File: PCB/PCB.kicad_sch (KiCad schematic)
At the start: 10 parts, among them J3 Conn_02x04_Odd_Even, J5 Conn_02x04_Odd_Even, U2 LM358

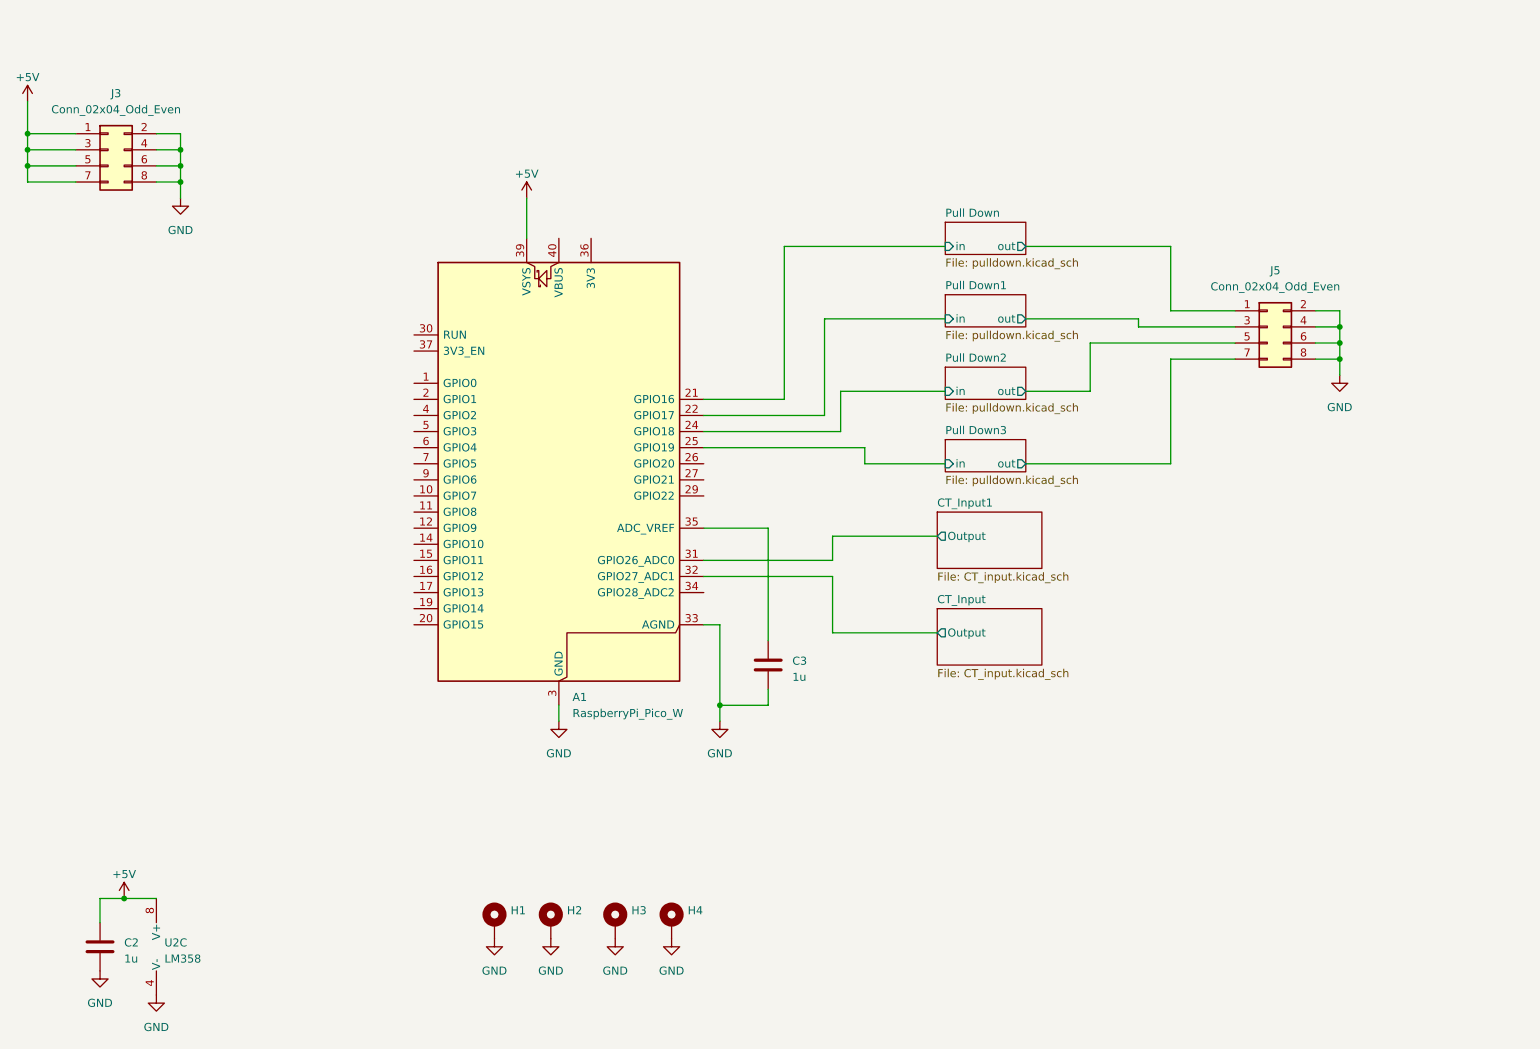
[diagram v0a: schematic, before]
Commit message: 1st draft PCB
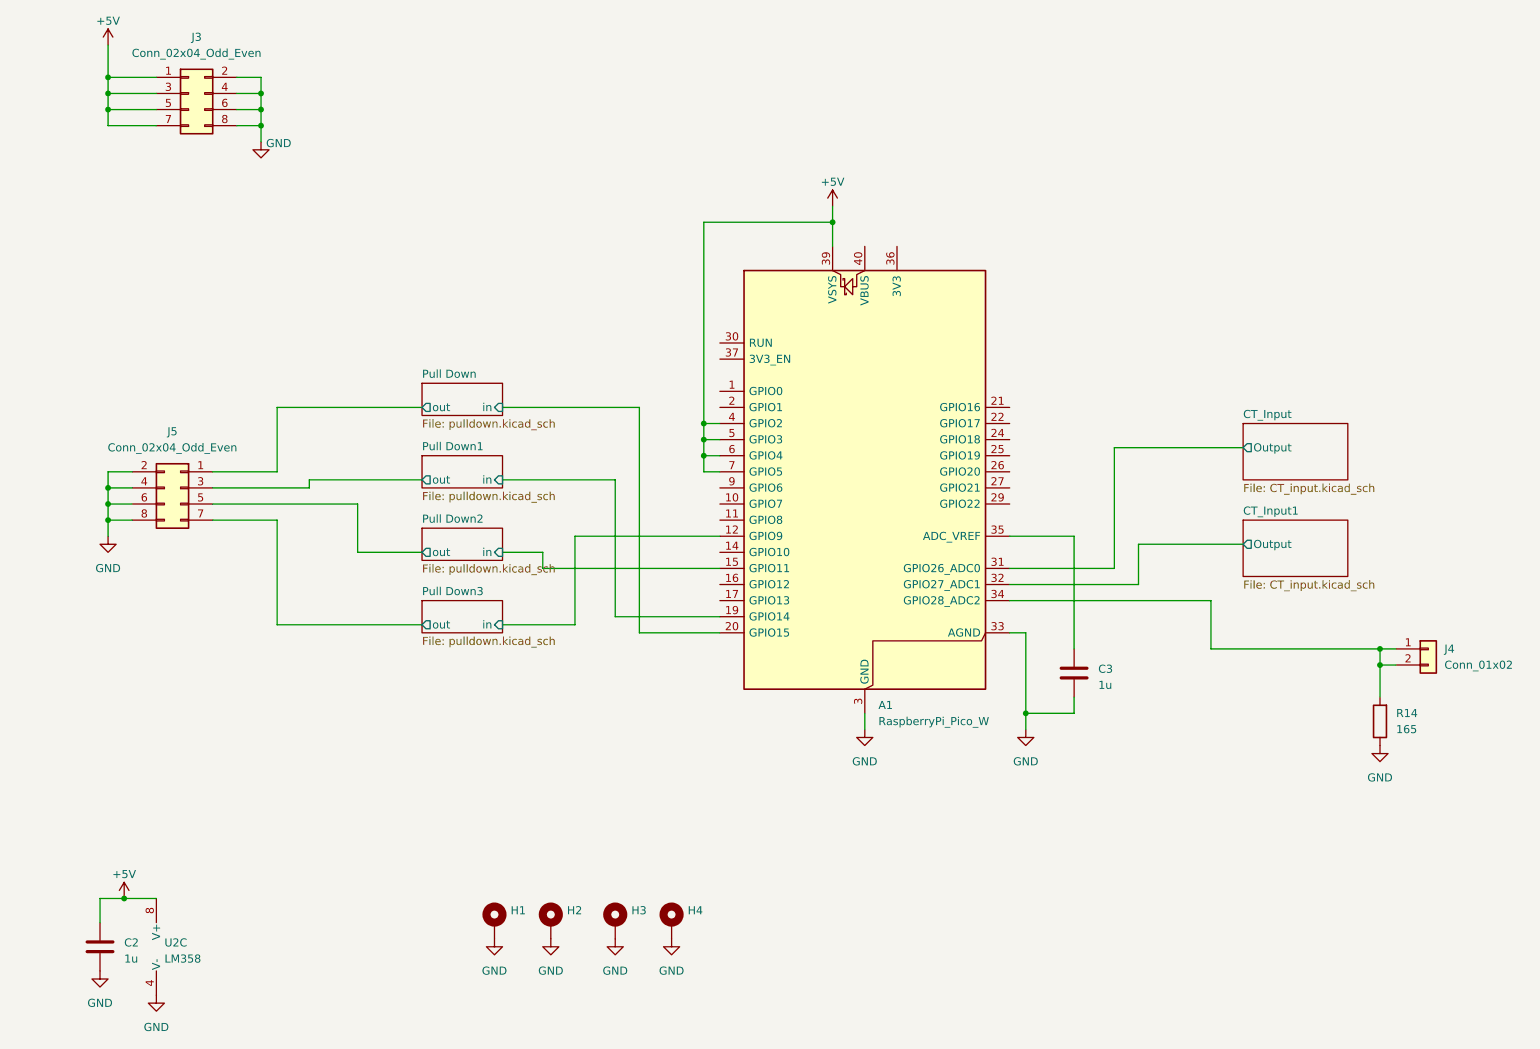
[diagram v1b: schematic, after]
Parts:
- added J4: Conn_01x02, Connector_PinHeader_2.54mm:PinHeader_1x02_P2.54mm_Vertical, symbol Connector_Generic:Conn_01x02
- added R14: 165, Resistor_SMD:R_0805_2012Metric_Pad1.20x1.40mm_HandSolder, symbol Device:R
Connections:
- net +5V: now also A1.4 (GPIO2), A1.5 (GPIO3), A1.6 (GPIO4), A1.7 (GPIO5)
- net CT_Input/Output: now also A1.31 (GPIO26_ADC0); no longer A1.32 (GPIO27_ADC1)
- net CT_Input1/Output: now also A1.32 (GPIO27_ADC1); no longer A1.31 (GPIO26_ADC0)
- net GND: now also R14.1
- net Pull Down/in: now also A1.20 (GPIO15); no longer A1.21 (GPIO16)
- net Pull Down1/in: now also A1.19 (GPIO14); no longer A1.22 (GPIO17)
- net Pull Down2/in: now also A1.15 (GPIO11); no longer A1.24 (GPIO18)
- net Pull Down3/in: now also A1.12 (GPIO9); no longer A1.25 (GPIO19)
- net at A1.34 (GPIO28_ADC2): now also J4.1 (Pin_1), J4.2 (Pin_2), R14.2
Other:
- moved on the sheet: A1, C3, J3, J5
